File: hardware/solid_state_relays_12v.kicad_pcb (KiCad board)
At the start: 2 copper layers, 100 x 90 mm, 86 parts, among them J1 1190297, J2 1190297, J3 1190297, J4 1190297, J5 1190297, J6 1190297, J7 1190297, J8 1190297, Q1 IRF4905PBF, Q2 IRF4905PBF, Q3 IRF4905PBF, Q4 IRF4905PBF, Q5 IRF4905PBF, Q6 IRF4905PBF, Q7 IRF4905PBF, Q8 IRF4905PBF

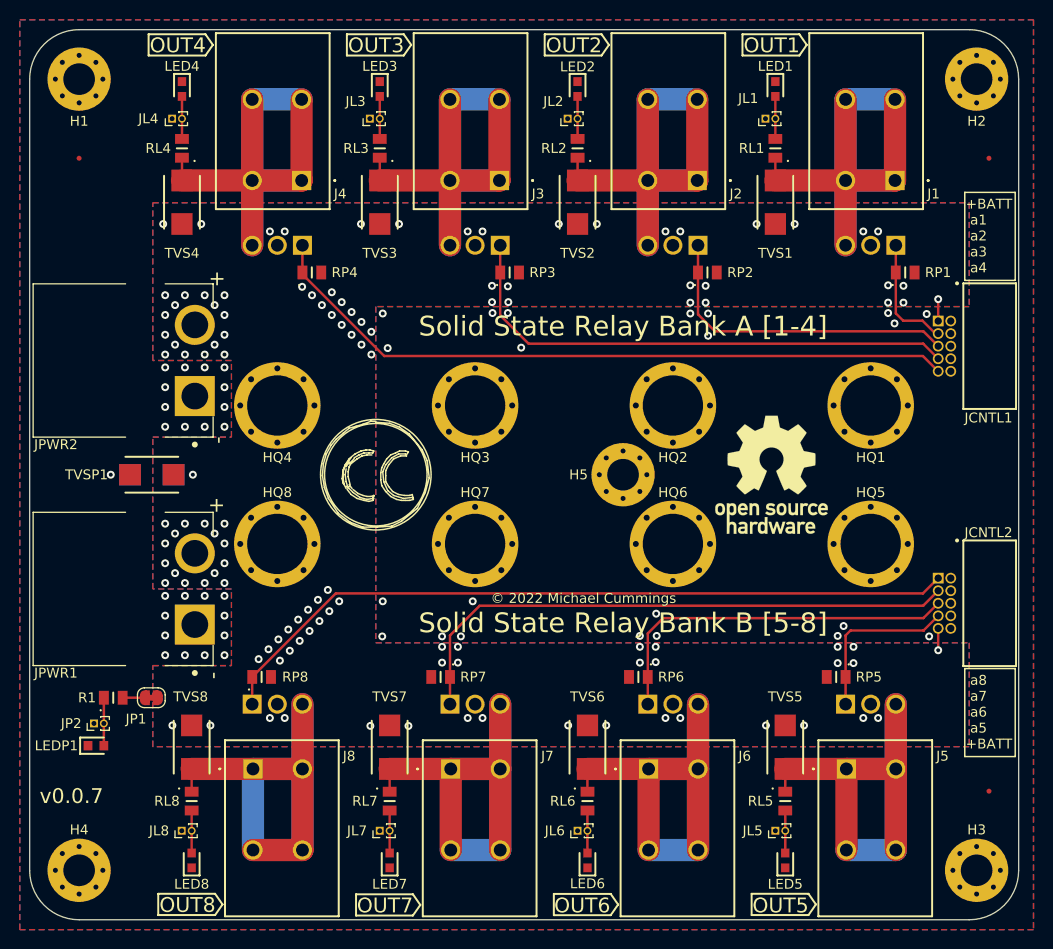
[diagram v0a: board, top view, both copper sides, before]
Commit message: Updated rev. to v0.0.8
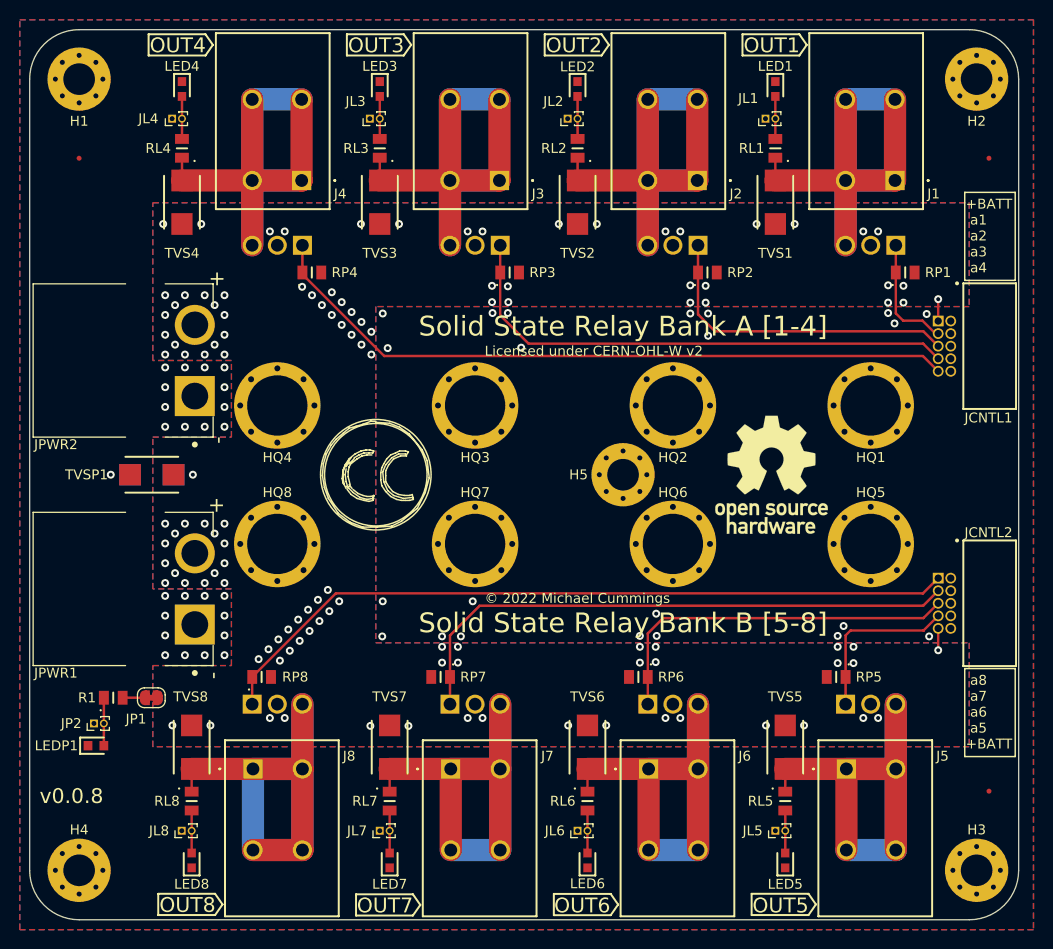
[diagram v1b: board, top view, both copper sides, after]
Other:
- board text added: "Licensed under CERN-OHL-W v2"
- board text added: "v0.0.8"
- board text removed: "v0.0.7"
